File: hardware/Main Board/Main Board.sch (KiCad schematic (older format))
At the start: 12 parts, among them J1 Daughter Board Connector, J2 ATtiny84 I2C/SPI Debug, J3 ATtiny85 I2c/SPI Debug, P1 Raspberry Pi, U1 ATtiny84-20PU, U2 ATtiny85-20PU

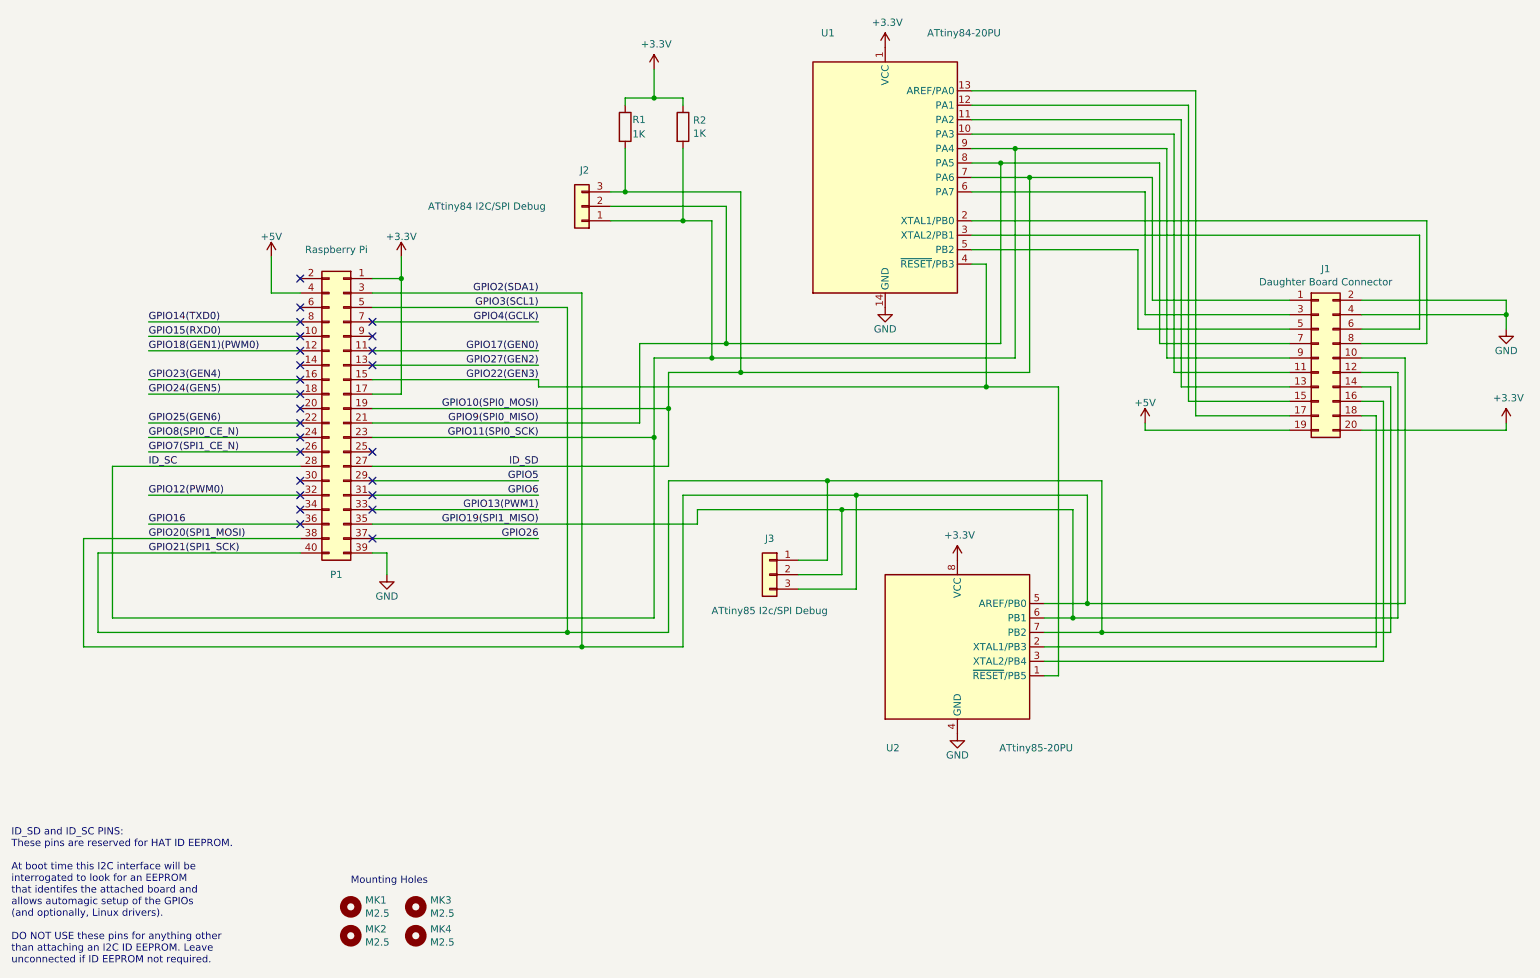
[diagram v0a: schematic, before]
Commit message: The New (v2) Board
Signed-off-by: John Jacques <eruditelite@gmail.com>
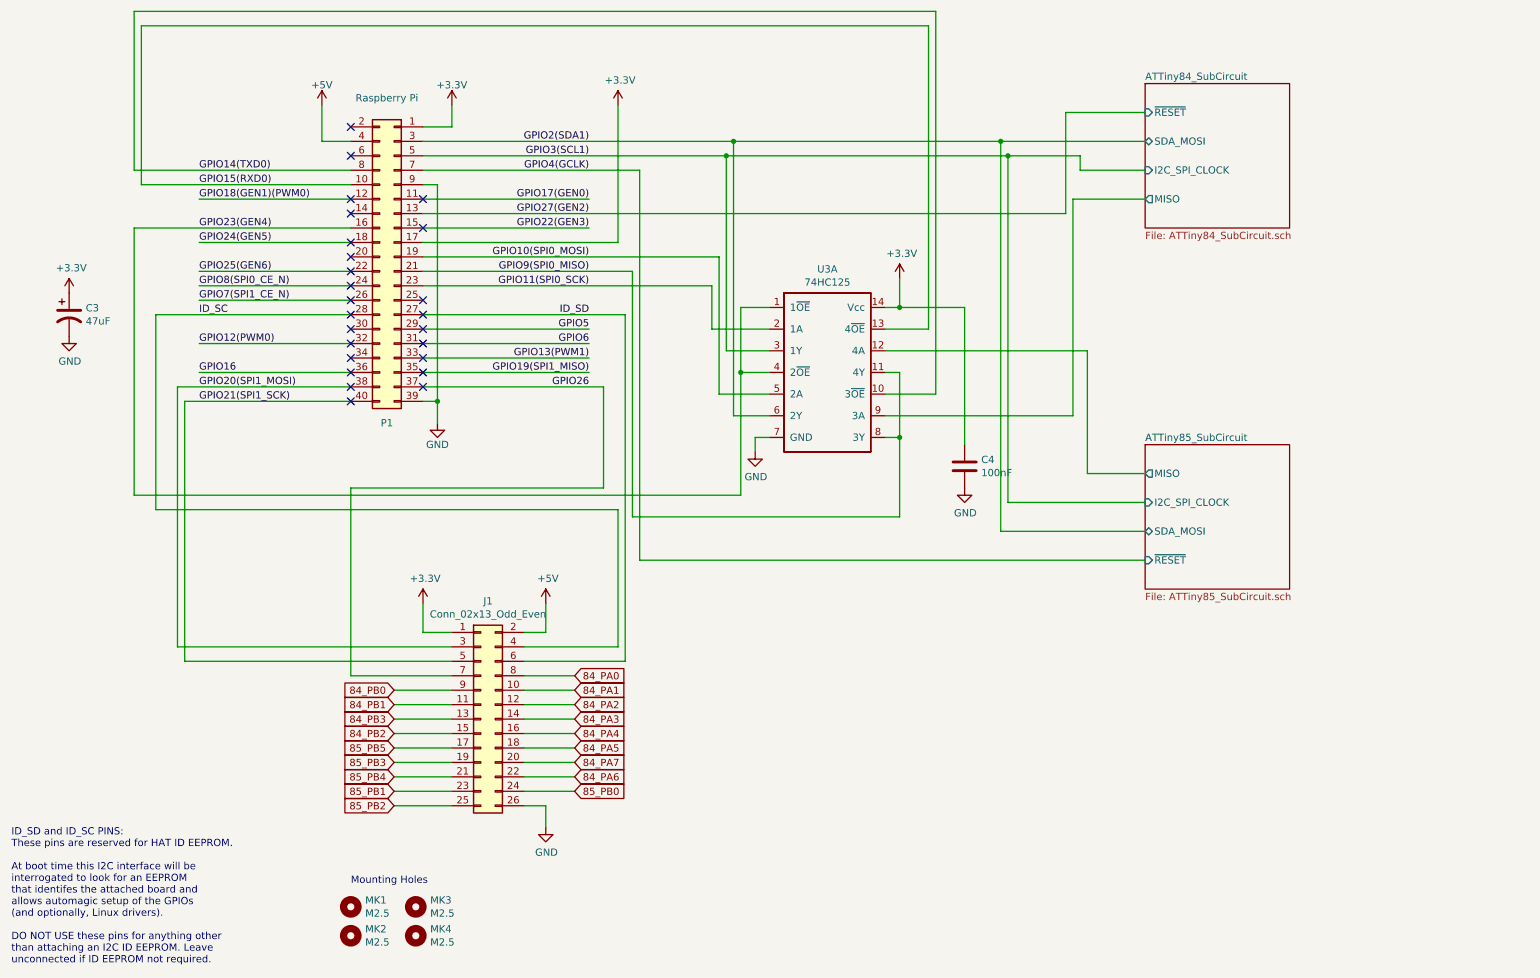
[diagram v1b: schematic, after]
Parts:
- removed J1: Daughter Board Connector, Connector_PinSocket_2.54mm:PinSocket_2x10_P2.54mm_Vertical, symbol Connector_Generic:Conn_02x10_Odd_Even
- removed J2: ATtiny84 I2C/SPI Debug, Connector_PinHeader_2.54mm:PinHeader_1x03_P2.54mm_Vertical, symbol Connector_Generic:Conn_01x03
- removed J3: ATtiny85 I2c/SPI Debug, Connector_PinHeader_2.54mm:PinHeader_1x03_P2.54mm_Vertical, symbol Connector_Generic:Conn_01x03
- removed R1, R2: 1K, Resistor_THT:R_Axial_DIN0207_L6.3mm_D2.5mm_P7.62mm_Horizontal, symbol Device:R
- removed U1: ATtiny84-20PU, Package_DIP:DIP-14_W7.62mm, symbol MCU_Microchip_ATtiny:ATtiny84-20PU
- removed U2: ATtiny85-20PU, Package_DIP:DIP-8_W7.62mm, symbol MCU_Microchip_ATtiny:ATtiny85-20PU
- added C3: 47uF, Capacitor_THT:CP_Radial_D6.3mm_P2.50mm, symbol Device:CP1
- added C4: 100nF, Capacitor_THT:C_Disc_D5.0mm_W2.5mm_P2.50mm, symbol Device:C
- added J1: Conn_02x13_Odd_Even, Connector_PinSocket_2.00mm:PinSocket_2x13_P2.00mm_Vertical, symbol Connector_Generic:Conn_02x13_Odd_Even
- added U3: 74HC125, Package_DIP:DIP-14_W7.62mm_Socket, symbol 74hc:74HC125
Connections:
- net +3V3: now also C3.1, C4.1, J1.1 (Pin_1), U3.14 (Vcc)
- net +5V: now also J1.2 (Pin_2)
- net GND: now also P1.9 (Pin_9), C3.2, C4.2, J1.26 (Pin_26), U3.7 (GND)
- net GPIO10(SPI0_MOSI): now also U3.5 (2A); no longer P1.27 (Pin_27)
- net GPIO11(SPI0_SCK): now also U3.2 (1A); no longer P1.28 (Pin_28)
- net GPIO14(TXD0): now also U3.10 (3~OE)
- net GPIO15(RXD0): now also U3.13 (4~OE)
- net GPIO2(SDA1): now also U3.6 (2Y); no longer P1.38 (Pin_38)
- net GPIO21(SPI1_SCK): now also J1.5 (Pin_5); no longer P1.5 (Pin_5)
- net GPIO23(GEN4): now also U3.1 (1~OE), U3.4 (2~OE)
- net GPIO26: now also J1.7 (Pin_7)
- net GPIO9(SPI0_MISO): now also U3.11 (4Y), U3.8 (3Y)
- new net 84_PA0: J1.8 (Pin_8)
- new net 84_PA1: J1.10 (Pin_10)
- new net 84_PA2: J1.12 (Pin_12)
- new net 84_PA3: J1.14 (Pin_14)
- new net 84_PA4: J1.16 (Pin_16)
- new net 84_PA5: J1.18 (Pin_18)
- new net 84_PA6: J1.22 (Pin_22)
- new net 84_PA7: J1.20 (Pin_20)
- new net 84_PB0: J1.9 (Pin_9)
- new net 84_PB1: J1.11 (Pin_11)
- new net 84_PB2: J1.15 (Pin_15)
- new net 84_PB3: J1.13 (Pin_13)
- new net 85_PB0: J1.24 (Pin_24)
- new net 85_PB1: J1.23 (Pin_23)
- new net 85_PB2: J1.25 (Pin_25)
- new net 85_PB3: J1.19 (Pin_19)
- new net 85_PB4: J1.21 (Pin_21)
- new net 85_PB5: J1.17 (Pin_17)
- new net ATTiny84_SubCircuit/MISO: U3.9 (3A)
- new net ATTiny85_SubCircuit/MISO: U3.12 (4A)
- new net GPIO20(SPI1_MOSI): J1.3 (Pin_3), P1.38 (Pin_38)
- new net GPIO3(SCL1): P1.5 (Pin_5), U3.3 (1Y)
- new net ID_SC: J1.4 (Pin_4), P1.28 (Pin_28)
- new net ID_SD: J1.6 (Pin_6), P1.27 (Pin_27)
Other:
- moved on the sheet: P1

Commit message: Fix an Error in the v2 Board
The custom footprint for the quad buffer had two pin 12s!
Updated the silk to release_2_1 as well.

Signed-off-by: John Jacques <eruditelite@gmail.com>
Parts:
- MK1, MK2, MK3, MK4: symbol Main-Board-rescue:Mounting_Hole-Mechanical-ATTiny-Examples-rescue -> PiMounts:Mounting_Hole-Mechanical
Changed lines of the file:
@@
 EESchema Schematic File Version 4
 LIBS:Main Board-cache
-EELAYER 29 0
+EELAYER 26 0
 EELAYER END
 $Descr A4 11693 8268
@@
 ID_SD and ID_SC PINS:\nThese pins are reserved for HAT ID EEPROM.\n\nAt boot time this I2C interface will be\ninterrogated to look for an EEPROM\nthat identifes the attached board and\nallows automagic setup of the GPIOs\n(and optionally, Linux drivers).\n\nDO NOT USE these pins for anything other\nthan attaching an I2C ID EEPROM. Leave\nunconnected if ID EEPROM not required.
 $Comp
-L Main-Board-rescue:Mounting_Hole-Mechanical-ATTiny-Examples-rescue MK1
+L PiMounts:Mounting_Hole-Mechanical MK1
 U 1 1 5834FB2E
 P 3000 7200
@@
 $EndComp
 $Comp
-L Main-Board-rescue:Mounting_Hole-Mechanical-ATTiny-Examples-rescue MK3
+L PiMounts:Mounting_Hole-Mechanical MK3
 U 1 1 5834FBEF
 P 3450 7200
@@
 $EndComp
 $Comp
-L Main-Board-rescue:Mounting_Hole-Mechanical-ATTiny-Examples-rescue MK2
+L PiMounts:Mounting_Hole-Mechanical MK2
 U 1 1 5834FC19
 P 3000 7400
@@
 $EndComp
 $Comp
-L Main-Board-rescue:Mounting_Hole-Mechanical-ATTiny-Examples-rescue MK4
+L PiMounts:Mounting_Hole-Mechanical MK4
 U 1 1 5834FC4F
 P 3450 7400
@@
 	5800 3950 5800 4050
 $Comp
-L Main_Board:GND #PWR02
+L Main-Board-rescue:GND-Main_Board-Main-Board-rescue #PWR02
 U 1 1 5CB3ADB4
 P 5800 4050
@@
 $EndComp
 $Comp
-L Main_Board:+3.3V #PWR07
+L Main-Board-rescue:+3.3V-Main_Board-Main-Board-rescue #PWR07
 U 1 1 5CB3DCF3
 P 6800 2850
@@
 	4850 2600 4850 1650
 $Comp
-L Main_Board:+3.3V #PWR0103
+L Main-Board-rescue:+3.3V-Main_Board-Main-Board-rescue #PWR0103
 U 1 1 5CB23E4A
 P 4850 1650
@@
 Connection ~ 6800 3050
 $Comp
-L Main_Board:GND #PWR016
+L Main-Board-rescue:GND-Main_Board-Main-Board-rescue #PWR016
 U 1 1 5CB26B05
 P 7250 4300
@@
 $EndComp
 $Comp
-L Main_Board:GND #PWR015
+L Main-Board-rescue:GND-Main_Board-Main-Board-rescue #PWR015
 U 1 1 5CB30D6E
 P 1050 3250
@@
 $EndComp
 $Comp
-L Main_Board:+3.3V #PWR014
+L Main-Board-rescue:+3.3V-Main_Board-Main-Board-rescue #PWR014
 U 1 1 5CB31393
 P 1050 2950
@@
 	4350 5300 4350 5100
 $Comp
-L Main_Board:+5V #PWR017
+L Main-Board-rescue:+5V-Main_Board-Main-Board-rescue #PWR017
 U 1 1 5CB47F57
 P 4350 5100
